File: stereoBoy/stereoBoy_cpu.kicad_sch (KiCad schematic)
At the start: 10 parts, among them J3 GameBoy_Cartridge, U2 RP2040, Y1 12M

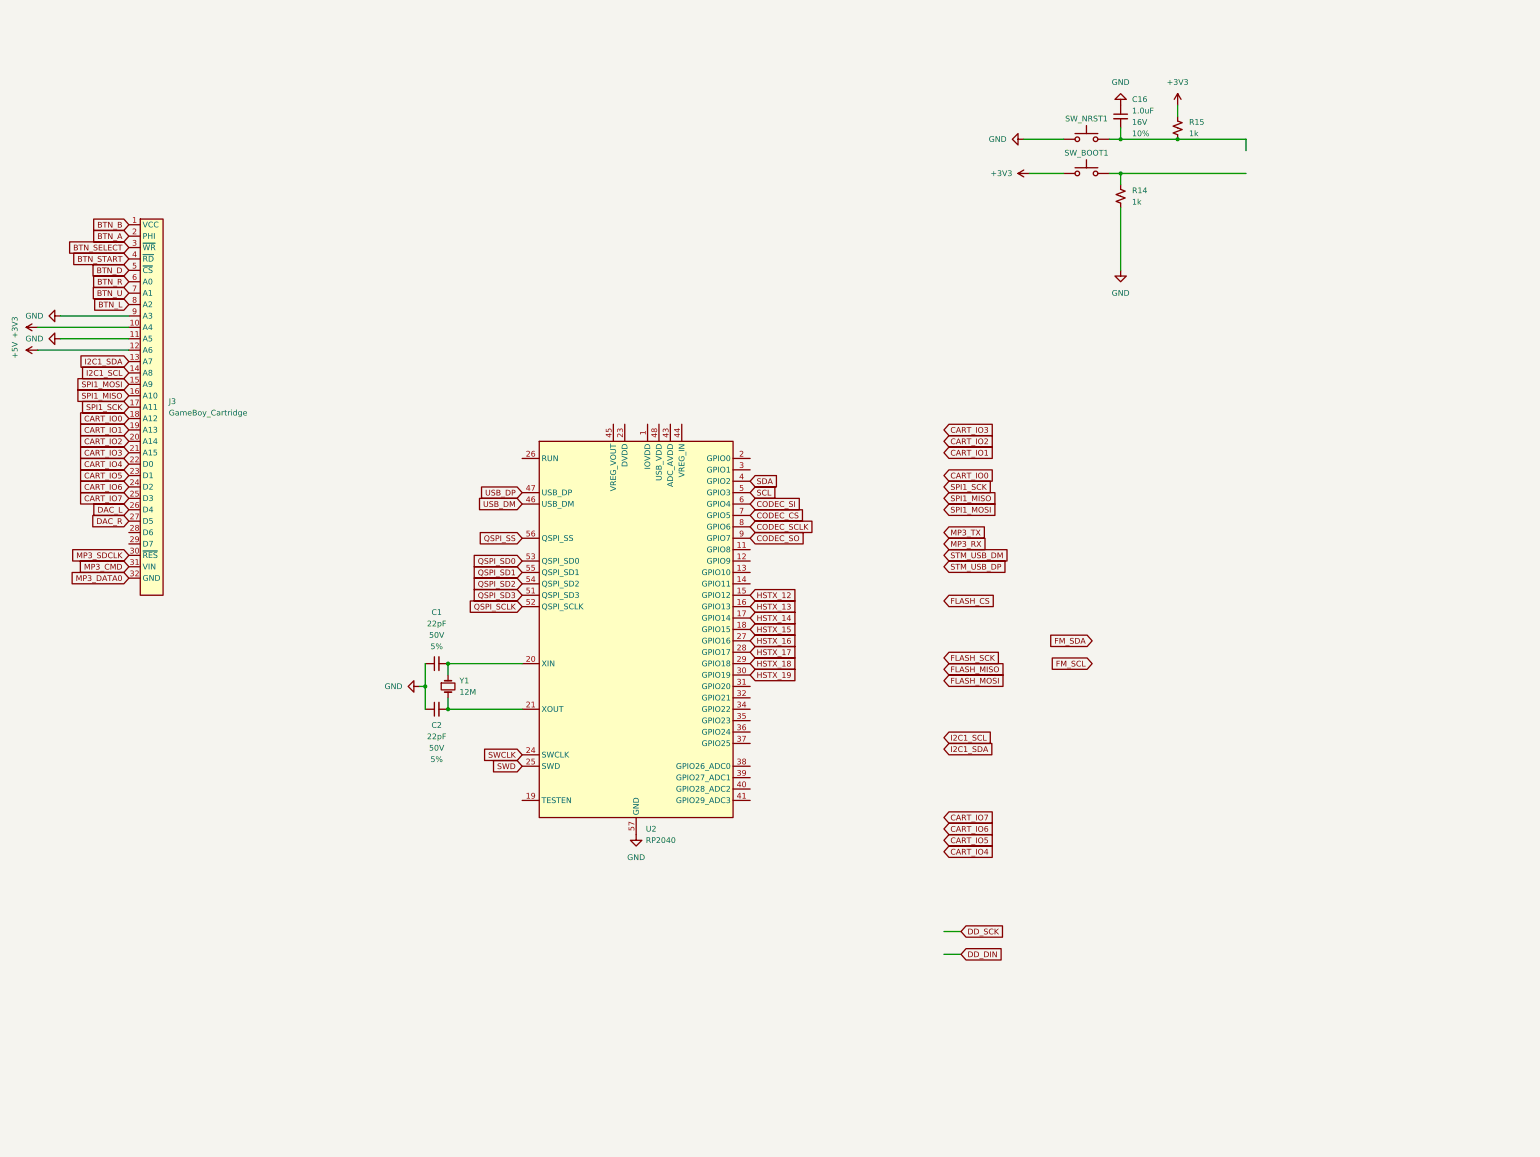
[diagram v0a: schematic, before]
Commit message: yeah
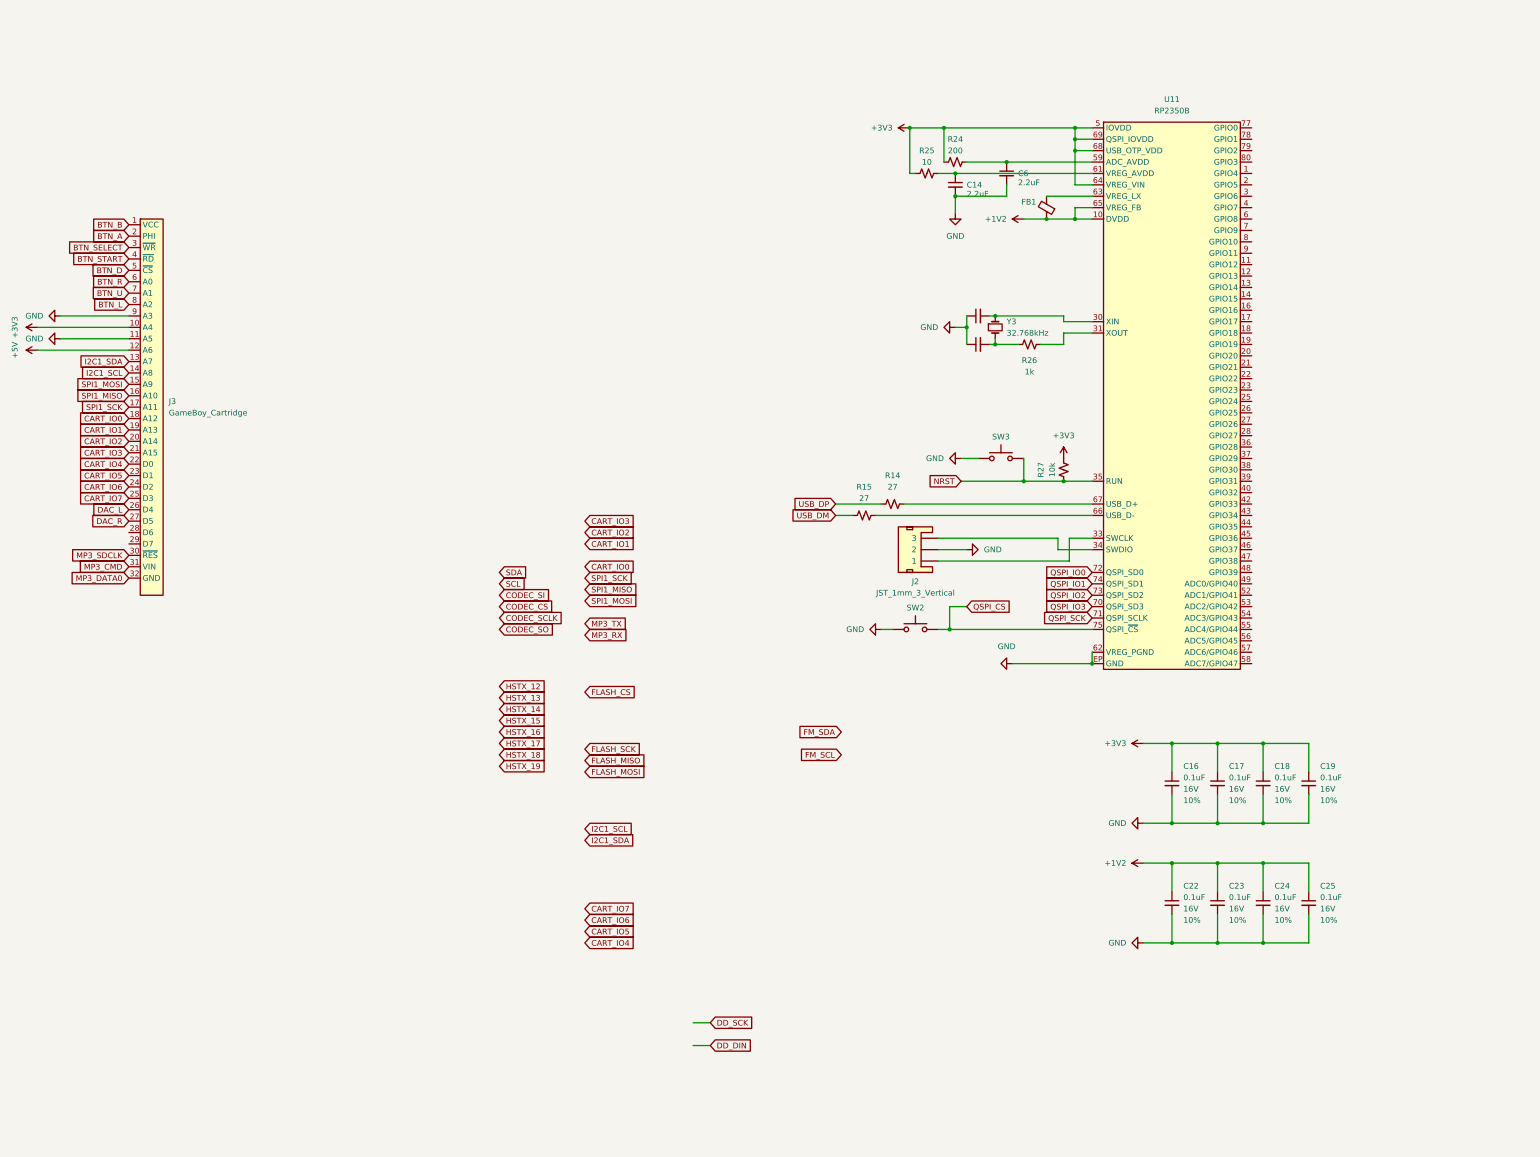
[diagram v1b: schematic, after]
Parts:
- removed C1, C2: 22pF, SparkFun-Capacitor:C_0402_1005Metric, symbol SparkFun-Capacitor:22pF_0402_50V_5%
- removed C16: 1.0uF, SparkFun-Capacitor:C_0603_1608Metric, symbol SparkFun-Capacitor:1.0uF_0603_16V_10%
- removed R14, R15: 1k, SparkFun-Resistor:R_0603_1608Metric, symbol SparkFun-Resistor:1k_0603
- removed SW_BOOT1, SW_NRST1: SMD_4.2x3.2mm_h2.5mm, SparkFun-Switch:Push_SMD_4.2x3.2mm, symbol SparkFun-Switch:SPST_Push_SMD_4.2x3.2mm_h2.5mm
- removed U2: RP2040, Package_DFN_QFN:QFN-56-1EP_7x7mm_P0.4mm_EP3.2x3.2mm, symbol MCU_RaspberryPi:RP2040
- removed Y1: 12M, SparkFun-Clock:Crystal_SMD_3.2x1.5mm, symbol SparkFun-Clock:Crystal_32.768kHz_3.2x1.5mm
- added C14, C6: 2.2uF, Capacitor_SMD:C_0402_1005Metric, symbol Device:C_Small
- added C16, C17, C18, C19, C22, C23, C24, C25: 0.1uF, SparkFun-Capacitor:C_0402_1005Metric, symbol SparkFun-Capacitor:0.1uF_0402_16V_10%
- added C20, C21: 18pF, SparkFun-Capacitor:C_0402_1005Metric, symbol SparkFun-Capacitor:18pF_0603_50V_5%
- added FB1: FerriteBead_Small, Inductor_SMD:L_0402_1005Metric, symbol Device:FerriteBead_Small
- added J2: JST_1mm_3_Vertical, SparkFun-Connector:JST_1x03_P1.0mm_Horizontal_SMD, symbol SparkFun-Connector:Conn_01x03_JST_P1.0mm_Vertical_SMD
- added R14, R15: 27, SparkFun-Resistor:R_0402_1005Metric, symbol SparkFun-Resistor:27_0603
- added R24: 200, Resistor_SMD:R_0402_1005Metric, symbol SparkFun-Resistor:330_0603
- added R25: 10, Resistor_SMD:R_0402_1005Metric, symbol SparkFun-Resistor:330_0603
- added R26: 1k, Resistor_SMD:R_0402_1005Metric, symbol SparkFun-Resistor:1k_0603
- added R27: 10k, Resistor_SMD:R_0603_1608Metric, symbol SparkFun-Resistor:330_0603
- added SW2, SW3: SMD_4.2x3.2mm_h2.5mm, SparkFun-Switch:Push_SMD_4.2x3.2mm, symbol SparkFun-Switch:SPST_Push_SMD_4.2x3.2mm_h2.5mm
- added U11: RP2350B, Package_DFN_QFN:QFN-80-1EP_10x10mm_P0.4mm_EP3.4x3.4mm, symbol SparkFun-IC-Microcontroller:RP2350B
- added Y3: 32.768kHz, SparkFun-Clock:Crystal_SMD_3.2x1.5mm, symbol SparkFun-Clock:Crystal_32.768kHz_3.2x1.5mm
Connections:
- net +3V3: now also C16.1, C17.1, C18.1, C19.1, R24.1, R25.1, R27.2, U11.15 (IOVDD), U11.24 (IOVDD), U11.29 (IOVDD), U11.41 (IOVDD), U11.5 (IOVDD), U11.50 (IOVDD), U11.60 (IOVDD), U11.64 (VREG_VIN), U11.68 (USB_OTP_VDD), U11.69 (QSPI_IOVDD), U11.76 (IOVDD)
- net GND: now also C14.2, C16.2, C17.2, C18.2, C19.2, C20.1, C21.1, C22.2, C23.2, C24.2, C25.2, C6.2, J2.2, SW2.1, SW3.1, U11.62 (VREG_PGND), U11.EP (GND)
- net USB_DM: now also R15.1
- net USB_DP: now also R14.1
- new net: C20.2, U11.30 (XIN), Y3.1
- new net: R26.2, U11.31 (XOUT)
- new net: J2.1, U11.33 (SWCLK)
- new net: J2.3, U11.34 (SWDIO)
- new net: C6.1, R24.2, U11.59 (ADC_AVDD)
- new net: C14.1, R25.2, U11.61 (VREG_AVDD)
- new net: FB1.2, U11.63 (VREG_LX)
- new net: R15.2, U11.66 (USB_D-)
- new net: R14.2, U11.67 (USB_D+)
- new net: C21.2, R26.1, Y3.2
- new net +1V2: C22.1, C23.1, C24.1, C25.1, FB1.1, U11.10 (DVDD), U11.32 (DVDD), U11.51 (DVDD), U11.65 (VREG_FB)
- new net NRST: R27.1, SW3.2, U11.35 (RUN)
- new net QSPI_CS: SW2.2, U11.75 (QSPI_~{CS})
- new net QSPI_IO0: U11.72 (QSPI_SD0)
- new net QSPI_IO1: U11.74 (QSPI_SD1)
- new net QSPI_IO2: U11.73 (QSPI_SD2)
- new net QSPI_IO3: U11.70 (QSPI_SD3)
- new net QSPI_SCK: U11.71 (QSPI_SCLK)

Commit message: yuh
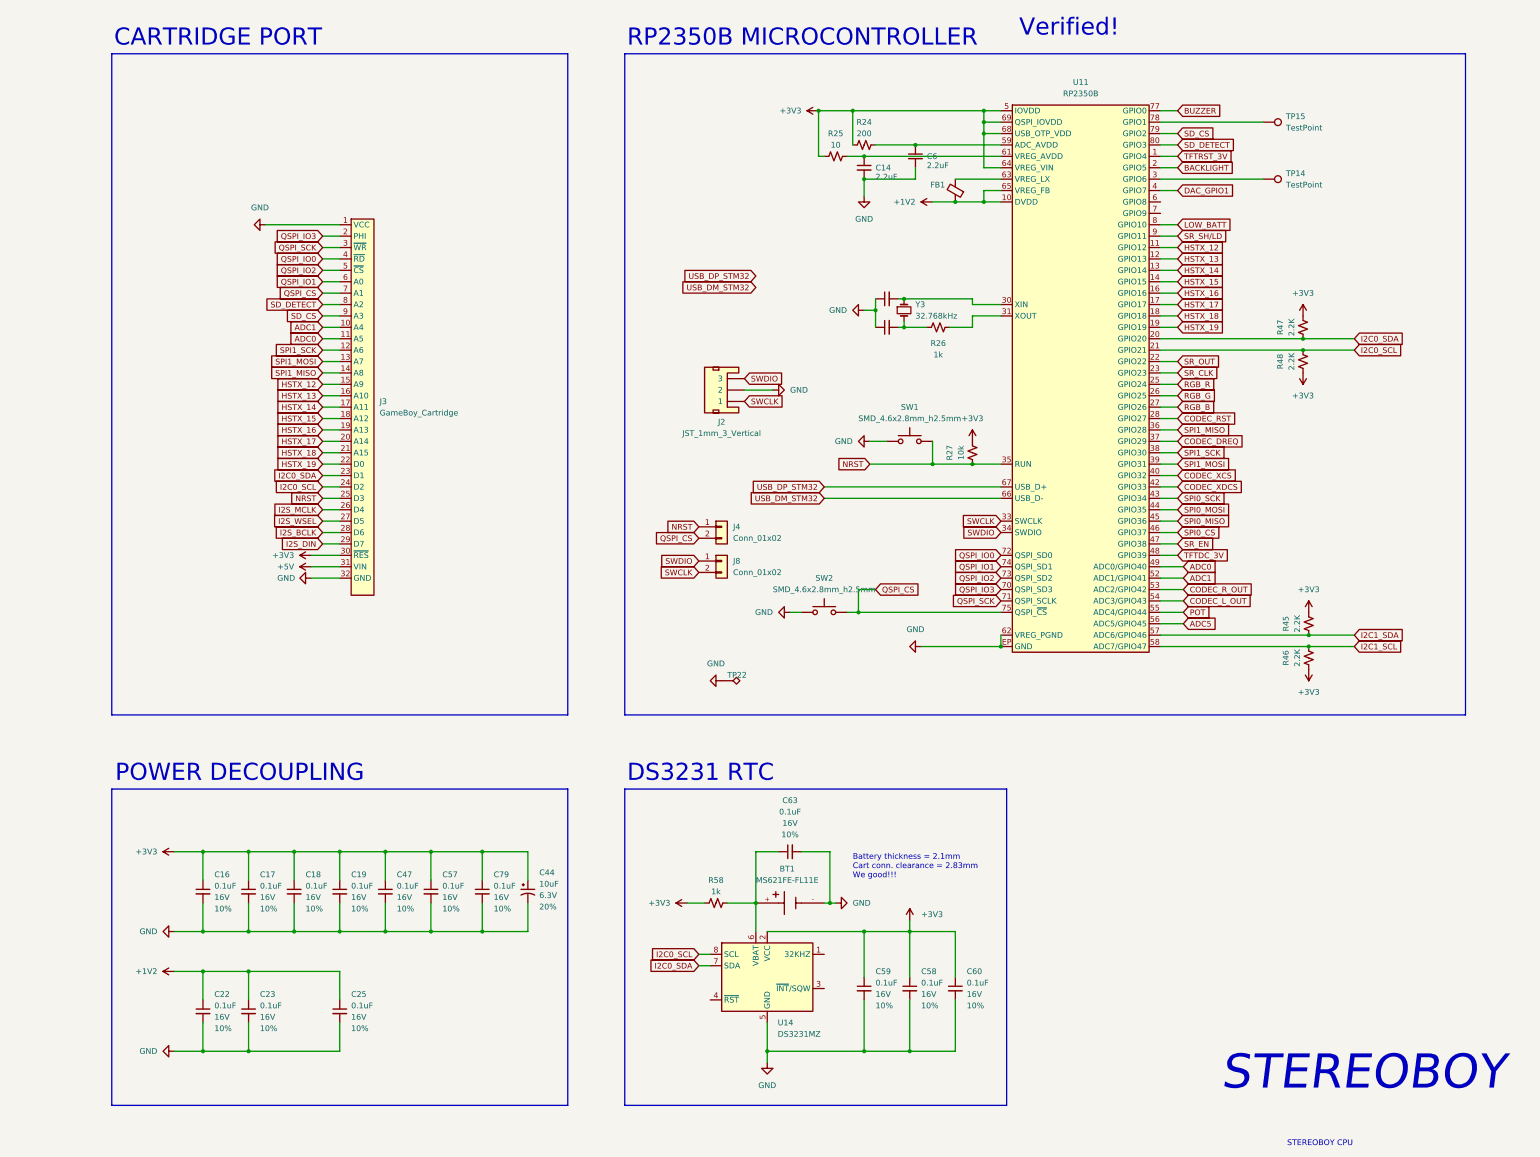
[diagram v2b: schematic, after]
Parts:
- removed C24: 0.1uF, SparkFun-Capacitor:C_0402_1005Metric, symbol SparkFun-Capacitor:0.1uF_0402_16V_10%
- removed R14, R15: 27, SparkFun-Resistor:R_0402_1005Metric, symbol SparkFun-Resistor:27_0603
- removed SW2, SW3: SMD_4.2x3.2mm_h2.5mm, SparkFun-Switch:Push_SMD_4.2x3.2mm, symbol SparkFun-Switch:SPST_Push_SMD_4.2x3.2mm_h2.5mm
- added BT1: MS621FE-FL11E, MS621FE_FL11E:MS621FE_FL11E, symbol MS621FE-FL11E:MS621FE-FL11E
- added C44: 10uF, Capacitor_SMD:CP_Elec_6.3x4.5, symbol SparkFun-Capacitor:10uF_0603_6.3V_20%_Polar(Tant)
- added C47, C57, C58, C60, C63, C79: 0.1uF, SparkFun-Capacitor:C_0402_1005Metric, symbol SparkFun-Capacitor:0.1uF_0402_16V_10%
- added C59: 0.1uF, SparkFun-Capacitor:C_0805_2012Metric, symbol SparkFun-Capacitor:0.1uF_0402_16V_10%
- added J4, J8: Conn_01x02, SparkFun-Connector:1x02_P2.54mm, symbol SparkFun-Connector:Conn_01x02_P2.54mm
- added R45, R46, R47, R48: 2.2K, Resistor_SMD:R_0402_1005Metric, symbol SparkFun-Resistor:330_0603
- added R58: 1k, Resistor_SMD:R_0402_1005Metric, symbol SparkFun-Resistor:330_0603
- added SW1, SW2: SMD_4.6x2.8mm_h2.5mm, SparkFun-Switch:Push_SMD_4.6x2.8mm_h2.5mm, symbol SparkFun-Switch:SPST_Push_SMD_4.6x2.8mm_h2.5mm
- added TP14, TP15: TestPoint, TestPoint:TestPoint_Pad_D1.0mm, symbol Connector:TestPoint
- added TP22: TestPoint_Alt, TestPoint:TestPoint_Pad_1.5x1.5mm, symbol Connector:TestPoint_Alt
- added U14: DS3231MZ, Package_SO:SOIC-8_3.9x4.9mm_P1.27mm, symbol Timer_RTC:DS3231MZ
- C20, C21: value 18pF -> 15pF
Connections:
- net BTN_A is gone; now on net QSPI_IO3: J3.2 (PHI)
- net BTN_B is gone; now on net GND: J3.1 (VCC)
- net BTN_D is gone; now on net QSPI_IO2: J3.5 (~{CS})
- net BTN_L is gone; now on net SD_DETECT: J3.8 (A2)
- net BTN_R is gone; now on net QSPI_IO1: J3.6 (A0)
- net BTN_SELECT is gone; now on net QSPI_SCK: J3.3 (~{WR})
- net BTN_START is gone; now on net QSPI_IO0: J3.4 (~{RD})
- net BTN_U is gone; now on net QSPI_CS: J3.7 (A1)
- net CART_IO0 is gone; now on net HSTX_15: J3.18 (A12)
- net CART_IO1 is gone; now on net HSTX_16: J3.19 (A13)
- net CART_IO2 is gone; now on net HSTX_17: J3.20 (A14)
- net CART_IO3 is gone; now on net HSTX_18: J3.21 (A15)
- net CART_IO4 is gone; now on net HSTX_19: J3.22 (D0)
- net CART_IO5 is gone; now on net I2C0_SDA: J3.23 (D1)
- net CART_IO6 is gone; now on net I2C0_SCL: J3.24 (D2)
- net CART_IO7 is gone; now on net NRST: J3.25 (D3)
- net MP3_CMD is gone; now on net +5V: J3.31 (VIN)
- net MP3_DATA0 is gone; now on net GND: J3.32 (GND)
- net MP3_SDCLK is gone; now on net +3V3: J3.30 (~{RES})
- net +3V3: now also C44.1, C47.1, C57.1, C58.1, C59.1, C60.1, C79.1, R45.2, R46.1, R47.2, R48.1, R58.1, U14.2 (VCC); no longer J3.10 (A4)
- net +5V: no longer J3.12 (A6)
- net GND: now also BT1.-, C44.2, C47.2, C57.2, C58.2, C59.2, C60.2, C63.2, C79.2, SW1.1, SW2.1, TP22.1, U14.5 (GND); no longer J3.11 (A5), J3.9 (A3)
- net HSTX_12: now also J3.15 (A9), U11.11 (GPIO12)
- net HSTX_13: now also J3.16 (A10), U11.12 (GPIO13)
- net HSTX_14: now also J3.17 (A11), U11.13 (GPIO14)
- net HSTX_15: now also U11.14 (GPIO15)
- net HSTX_16: now also U11.16 (GPIO16)
- net HSTX_17: now also U11.17 (GPIO17)
- net HSTX_18: now also U11.18 (GPIO18)
- net HSTX_19: now also U11.19 (GPIO19)
- net I2C1_SCL: now also U11.58 (ADC7/GPIO47), R46.2; no longer J3.14 (A8)
- net I2C1_SDA: now also U11.57 (ADC6/GPIO46), R45.1; no longer J3.13 (A7)
- net NRST: now also J4.1 (Pin_1), SW1.2
- net QSPI_CS: now also J4.2 (Pin_2), SW2.2
- net SPI1_MISO: now also J3.14 (A8), U11.36 (GPIO28); no longer J3.16 (A10)
- net SPI1_MOSI: now also J3.13 (A7), U11.39 (GPIO31); no longer J3.15 (A9)
- net SPI1_SCK: now also J3.12 (A6), U11.38 (GPIO30); no longer J3.17 (A11)
- net TFTRST_3V: now reaches U11.1 (GPIO4)
- net BACKLIGHT: now reaches U11.2 (GPIO5)
- net I2C0_SDA: now reaches U11.20 (GPIO20)
- net I2C0_SDA: now also R47.1, U14.7 (SDA)
- net I2C0_SCL: now reaches U11.21 (GPIO21)
- net I2C0_SCL: now also R48.2, U14.8 (SCL)
- net SR_OUT: now reaches U11.22 (GPIO22)
- net SR_CLK: now reaches U11.23 (GPIO23)
- net RGB_R: now reaches U11.25 (GPIO24)
- net RGB_G: now reaches U11.26 (GPIO25)
- net RGB_B: now reaches U11.27 (GPIO26)
- net CODEC_RST: now reaches U11.28 (GPIO27)
- net at U11.3 (GPIO6): now also TP14.1
- net SWCLK: now reaches J2.1, U11.33 (SWCLK)
- net SWCLK: now also J8.2 (Pin_2)
- net SWDIO: now reaches J2.3, U11.34 (SWDIO)
- net SWDIO: now also J8.1 (Pin_1)
- net CODEC_DREQ: now reaches U11.37 (GPIO29)
- net DAC_GPIO1: now reaches U11.4 (GPIO7)
- net CODEC_XCS: now reaches U11.40 (GPIO32)
- net CODEC_XDCS: now reaches U11.42 (GPIO33)
- net SPI0_SCK: now reaches U11.43 (GPIO34)
- net SPI0_MOSI: now reaches U11.44 (GPIO35)
- net SPI0_MISO: now reaches U11.45 (GPIO36)
- net SPI0_CS: now reaches U11.46 (GPIO37)
- net SR_EN: now reaches U11.47 (GPIO38)
- net TFTDC_3V: now reaches U11.48 (GPIO39)
- net ADC0: now reaches U11.49 (ADC0/GPIO40)
- net ADC0: now also J3.11 (A5)
- net ADC1: now reaches U11.52 (ADC1/GPIO41)
- net ADC1: now also J3.10 (A4)
- net CODEC_R_OUT: now reaches U11.53 (ADC2/GPIO42)
- net CODEC_L_OUT: now reaches U11.54 (ADC3/GPIO43)
- net POT: now reaches U11.55 (ADC4/GPIO44)
- net ADC5: now reaches U11.56 (ADC5/GPIO45)
- net USB_DM_STM32: now reaches U11.66 (USB_D-)
- net USB_DP_STM32: now reaches U11.67 (USB_D+)
- net BUZZER: now reaches U11.77 (GPIO0)
- net at U11.78 (GPIO1): now also TP15.1
- net SD_CS: now reaches U11.79 (GPIO2)
- net SD_CS: now also J3.9 (A3)
- net LOW_BATT: now reaches U11.8 (GPIO10)
- net SD_DETECT: now reaches U11.80 (GPIO3)
- net SR_SH/LD: now reaches U11.9 (GPIO11)
- net I2S_BCLK: now reaches J3.28 (D6)
- net I2S_DIN: now reaches J3.29 (D7)
- net DAC_L renamed I2S_MCLK
- net DAC_R renamed I2S_WSEL
- new net: BT1.+, C63.1, R58.2, U14.6 (VBAT)
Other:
- note added: "Battery thickness = 2.1mm Cart conn. clearance = 2.83mm We good!!!"
- note added: "CARTRIDGE PORT"
- note added: "DS3231 RTC"
- note added: "POWER DECOUPLING"
- note added: "RP2350B MICROCONTROLLER"
- note added: "STEREOBOY"
- note added: "STEREOBOY CPU"
- note added: "Verified!"
- moved on the sheet: C14, C16, C17, C18, C19, C22, C23, C25, C6, FB1, J2, J3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
